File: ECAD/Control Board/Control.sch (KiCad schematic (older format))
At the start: 1 part

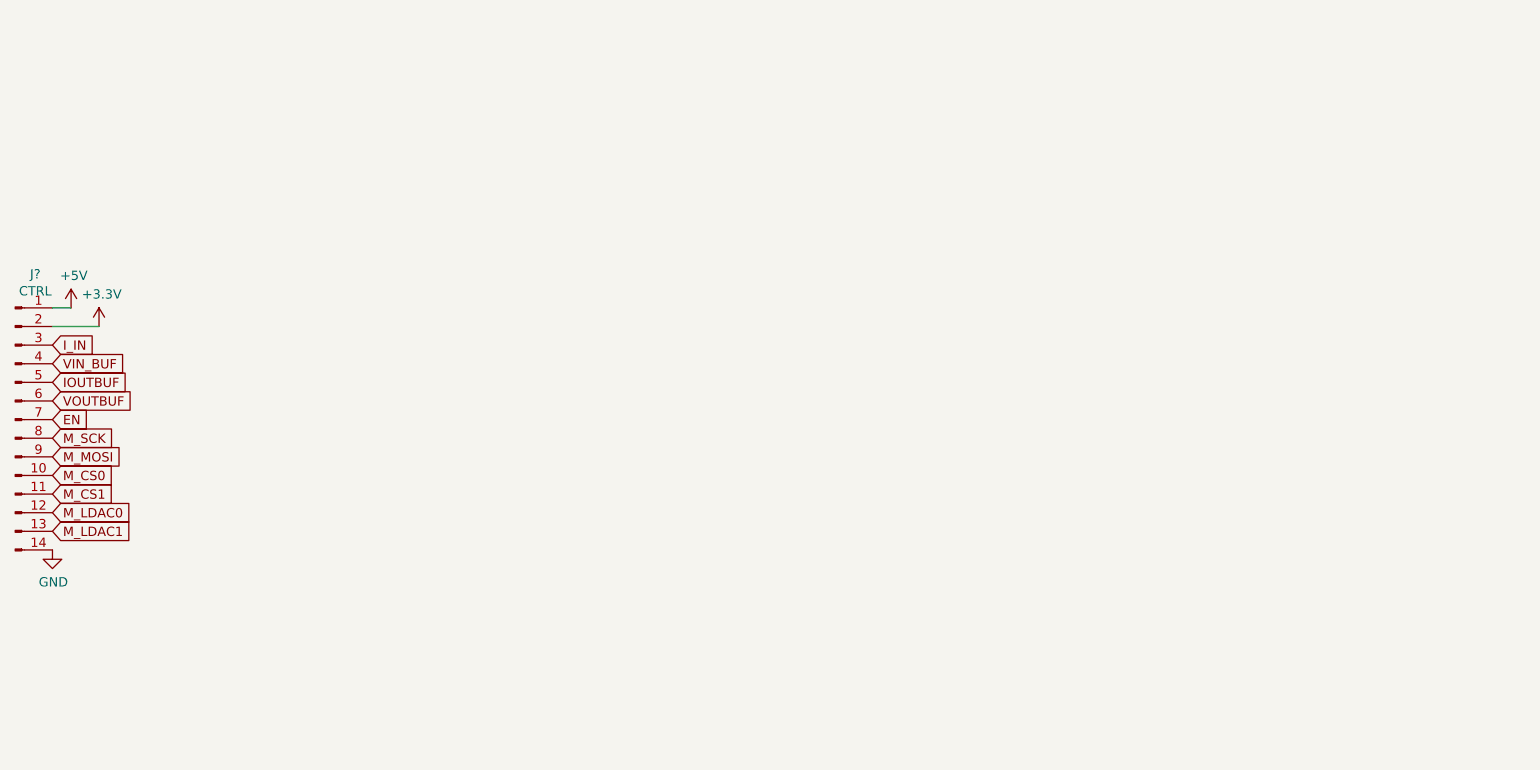
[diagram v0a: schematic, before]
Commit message: control
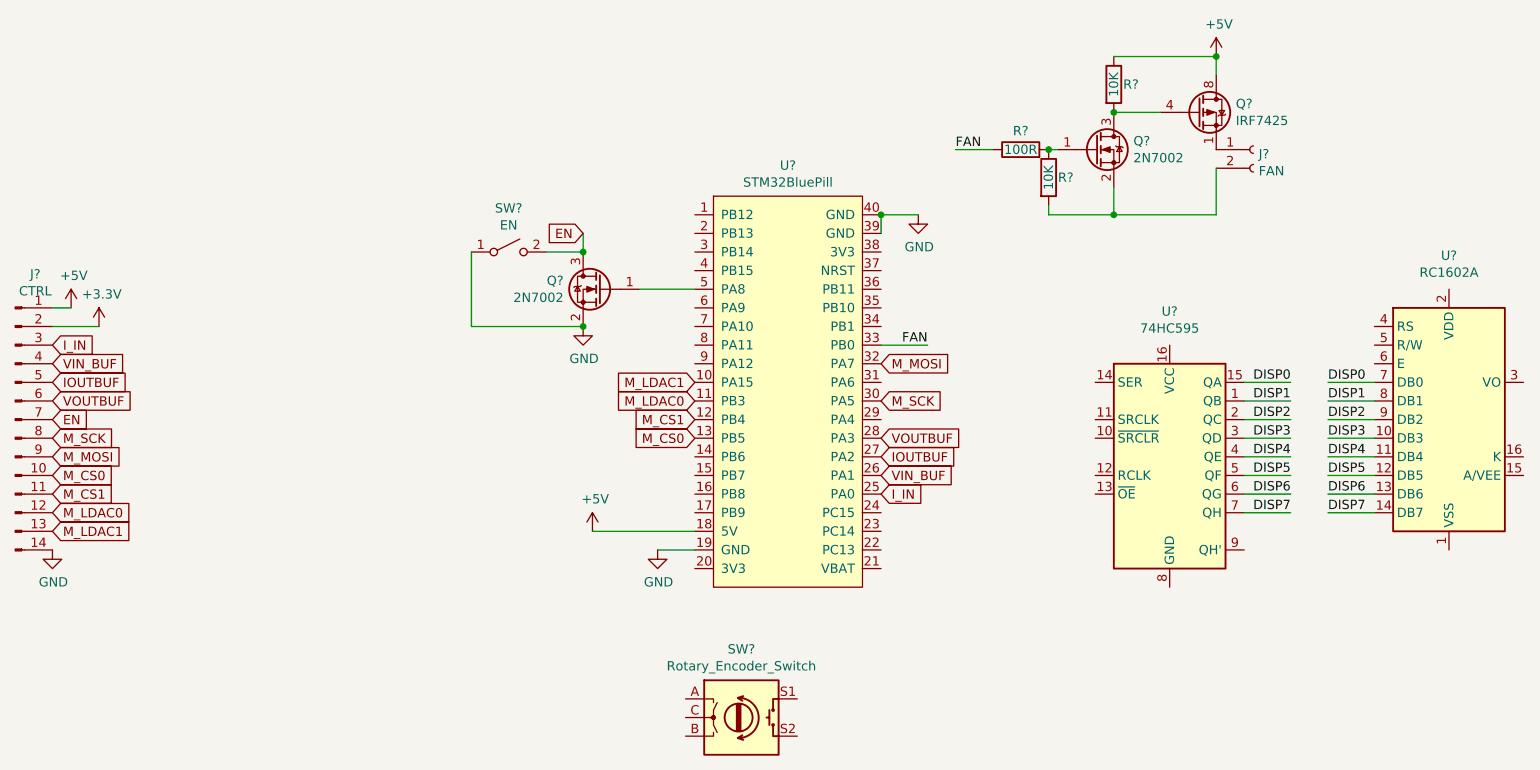
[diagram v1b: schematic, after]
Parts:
- added J?: FAN, symbol Connector:Conn_01x02_Female
- added Q? (x2): 2N7002, Package_TO_SOT_SMD:SOT-23, symbol Transistor_FET:2N7002
- added Q?: IRF7425, Package_SO:SOIC-8_3.9x4.9mm_P1.27mm, symbol Transistor_FET:IRF7404
- added R? (x2): 10K, symbol Device:R
- added R?: 100R, symbol Device:R
- added SW?: EN, symbol Switch:SW_SPST
- added SW?: Rotary_Encoder_Switch, symbol Device:Rotary_Encoder_Switch
- added U?: STM32BluePill, symbol symbols:STM32BluePill
- added U?: RC1602A, Display:RC1602A, symbol Display_Character:RC1602A
- added U?: 74HC595, symbol 74xx:74HC595
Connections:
- net +5V: now also Q?.5 (D), Q?.6 (D), Q?.7 (D), Q?.8 (D), R?.1, U?.18 (5V)
- net EN: now also Q?.3 (D), SW?.2 (B)
- net GND: now also Q?.2 (S), SW?.1 (A), U?.19 (GND), U?.39 (GND), U?.40 (GND)
- net IOUTBUF: now also U?.27 (PA2)
- net I_IN: now also U?.25 (PA0)
- net M_CS0: now also U?.13 (PB5)
- net M_CS1: now also U?.12 (PB4)
- net M_LDAC0: now also U?.11 (PB3)
- net M_LDAC1: now also U?.10 (PA15)
- net M_MOSI: now also U?.32 (PA7)
- net M_SCK: now also U?.30 (PA5)
- net VIN_BUF: now also U?.26 (PA1)
- net VOUTBUF: now also U?.28 (PA3)
- new net: Q?.1 (G), U?.5 (PA8)
- new net: J?.1 (Pin_1), Q?.1 (S), Q?.2 (S), Q?.3 (S)
- new net: Q?.3 (D), Q?.4 (G), R?.2
- new net: J?.2 (Pin_2), Q?.2 (S), R?.2
- new net: Q?.1 (G), R?.1, R?.2
- new net DISP0: U?.15 (QA), U?.7 (DB0)
- new net DISP1: U?.1 (QB), U?.8 (DB1)
- new net DISP2: U?.2 (QC), U?.9 (DB2)
- new net DISP3: U?.10 (DB3), U?.3 (QD)
- new net DISP4: U?.11 (DB4), U?.4 (QE)
- new net DISP5: U?.12 (DB5), U?.5 (QF)
- new net DISP6: U?.13 (DB6), U?.6 (QG)
- new net DISP7: U?.14 (DB7), U?.7 (QH)
- new net FAN: R?.1, U?.33 (PB0)
